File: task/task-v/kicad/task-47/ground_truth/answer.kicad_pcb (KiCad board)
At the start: 2 copper layers, 65 x 56.5 mm, 5 parts

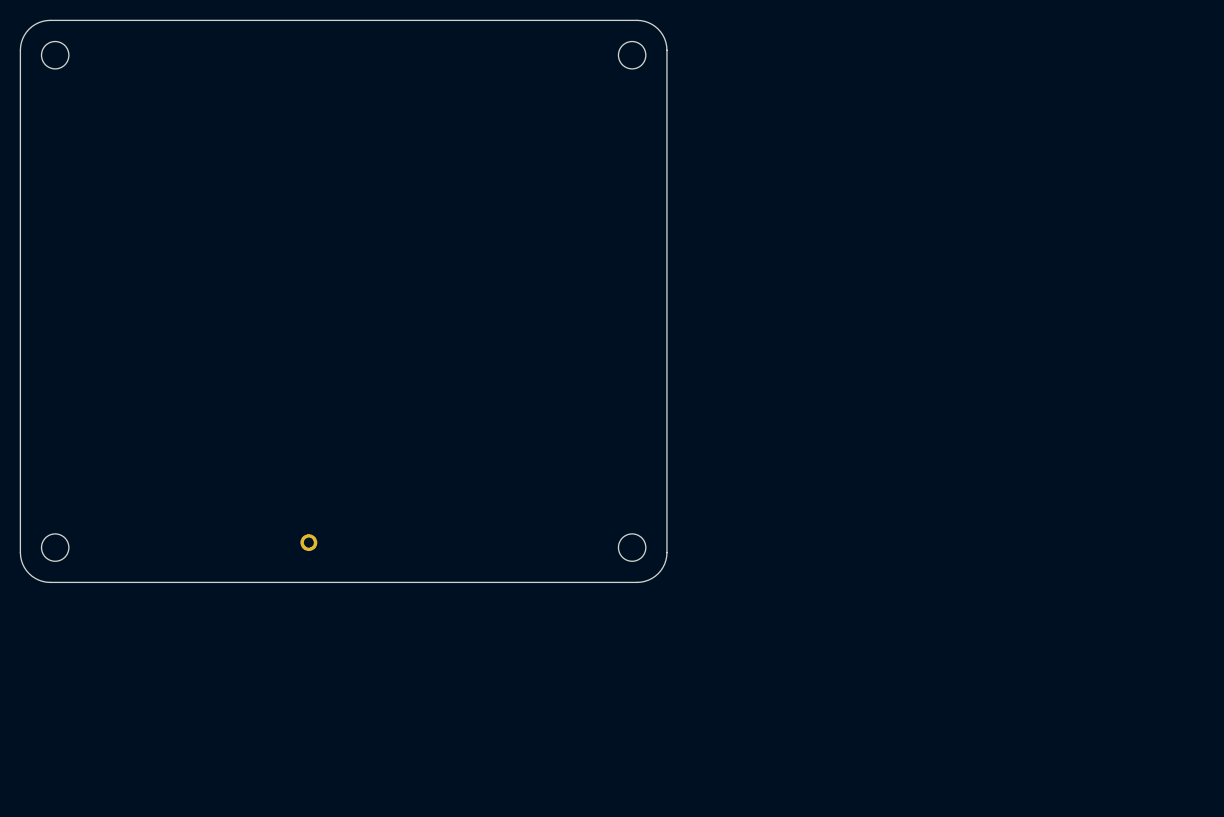
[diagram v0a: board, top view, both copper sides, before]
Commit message: Refine engineering task metadata and instructions
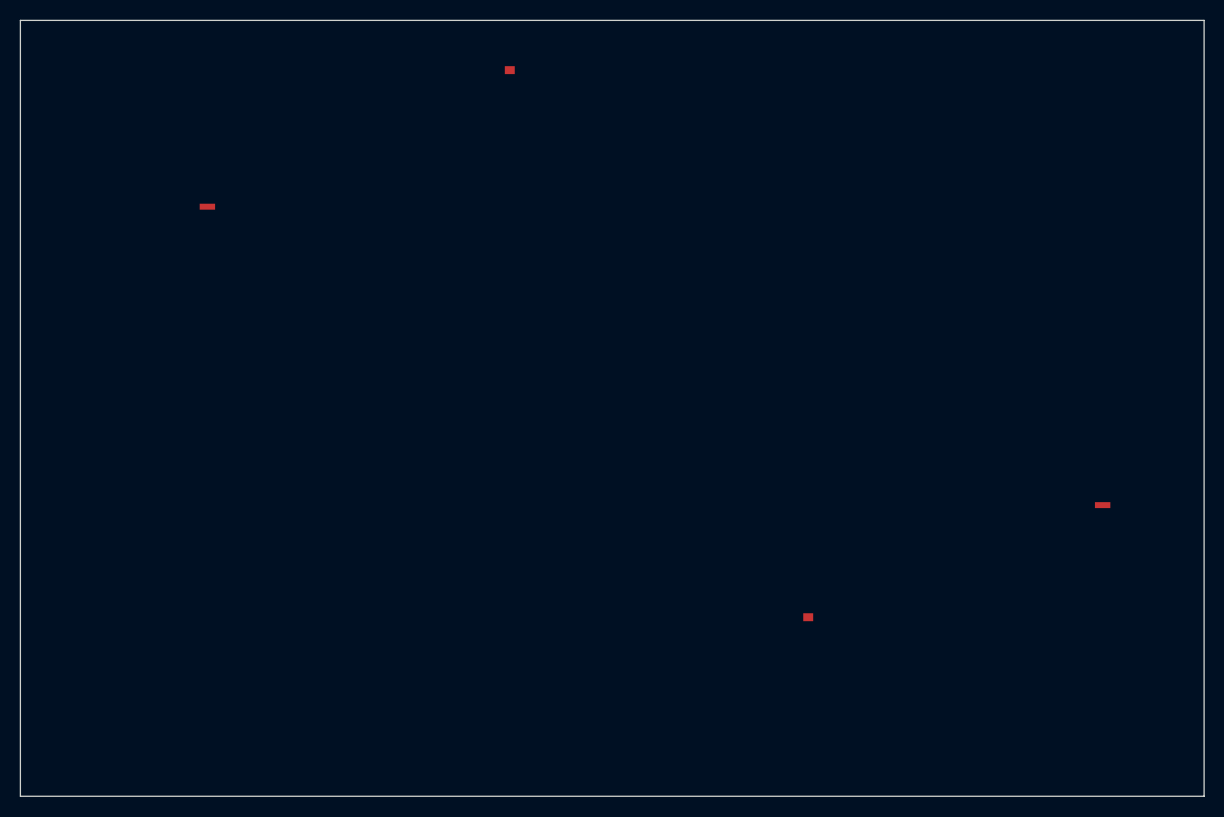
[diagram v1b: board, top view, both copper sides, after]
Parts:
- removed the ? at (3.50, 3.50)
- removed the ? at (61.5, 3.50)
- removed the ? at (3.50, 53.0)
- removed the ? at (61.5, 53.0)
- removed the ? at (29.0, 52.5)
- added ?: , Package_SO:SOIC-8_3.9x4.9mm_P1.27mm, F.Cu at (20.0, 20.0)
- added ?: , Resistor_SMD:R_0603_1608Metric, F.Cu at (50.0, 5.00)
- added ?: , Package_SO:SOIC-8_3.9x4.9mm_P1.27mm, F.Cu at (110.0, 50.0)
- added ?: , Resistor_SMD:R_0603_1608Metric, F.Cu at (80.0, 60.0)
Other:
- board size 65 x 56.5 mm -> 119 x 78 mm
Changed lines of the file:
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@@
   (net 1 "VCC")
   (net 2 "GND")
-  ; HAT+ board outline: 65x56.5mm with R=3mm rounded corners
-  ; Straight edges
-  (gr_line (start 3 0) (end 62 0) (layer "Edge.Cuts") (width 0.1))
-  (gr_line (start 65 3) (end 65 53.5) (layer "Edge.Cuts") (width 0.1))
-  (gr_line (start 62 56.5) (end 3 56.5) (layer "Edge.Cuts") (width 0.1))
-  (gr_line (start 0 53.5) (end 0 3) (layer "Edge.Cuts") (width 0.1))
-  ; Rounded corners (gr_arc: start, mid, end)
-  ; Bottom-left corner: center(3,3), R=3, arc from (0,3) through (0.879,0.879) to (3,0)
-  (gr_arc (start 0 3) (mid 0.879 0.879) (end 3 0) (layer "Edge.Cuts") (width 0.1))
-  ; Bottom-right corner: center(62,3), R=3, arc from (62,0) through (64.121,0.879) to (65,3)
-  (gr_arc (start 62 0) (mid 64.121 0.879) (end 65 3) (layer "Edge.Cuts") (width 0.1))
-  ; Top-right corner: center(62,53.5), R=3, arc from (65,53.5) through (64.121,55.621) to (62,56.5)
-  (gr_arc (start 65 53.5) (mid 64.121 55.621) (end 62 56.5) (layer "Edge.Cuts") (width 0.1))
-  ; Top-left corner: center(3,53.5), R=3, arc from (3,56.5) through (0.879,55.621) to (0,53.5)
-  (gr_arc (start 3 56.5) (mid 0.879 55.621) (end 0 53.5) (layer "Edge.Cuts") (width 0.1))
-  ; 4 M2.5 mounting holes at HAT+ spec positions
-  (footprint "MountingHole:MountingHole_2.75mm_M2.5" (layer "F.Cu") (at 3.5 3.5)
-    (reference "H1") (value "MountingHole")
-    (pad "" np_thru_hole circle (at 0 0) (size 2.75 2.75) (drill 2.75)
-      (layers "F.Cu" "B.Cu" "F.Mask" "B.Mask"))
+  ; Shrunk board: 119x78mm to fit Hammond 1455C1201 slot
+  (gr_rect (start 0 0) (end 119 78) (layer "Edge.Cuts") (width 0.1))
+  ; U1 at (20,20): dist to edges = min(20,99,20,58) = 20mm >= 3mm ✓
+  (footprint "Package_SO:SOIC-8_3.9x4.9mm_P1.27mm" (layer "F.Cu") (at 20 20)
+    (reference "U1") (value "OPAMP")
+    (pad "1" smd rect (at -1.2 -1.27) (size 1.55 0.6)
+      (layers "F.Cu" "F.Paste" "F.Mask") (net 1 "VCC"))
   )
-  (footprint "MountingHole:MountingHole_2.75mm_M2.5" (layer "F.Cu") (at 61.5 3.5)
-    (reference "H2") (value "MountingHole")
-    (pad "" np_thru_hole circle (at 0 0) (size 2.75 2.75) (drill 2.75)
-      (layers "F.Cu" "B.Cu" "F.Mask" "B.Mask"))
+  ; R1 moved from (50,1.5) to (50,5): dist to bottom edge = 5mm >= 3mm ✓
+  (footprint "Resistor_SMD:R_0603_1608Metric" (layer "F.Cu") (at 50 5)
+    (reference "R1") (value "4.7k")
+    (pad "1" smd rect (at -0.8 0) (size 1.0 0.8)
+      (layers "F.Cu" "F.Paste" "F.Mask") (net 1 "VCC"))
   )
-  (footprint "MountingHole:MountingHole_2.75mm_M2.5" (layer "F.Cu") (at 3.5 53)
-    (reference "H3") (value "MountingHole")
-    (pad "" np_thru_hole circle (at 0 0) (size 2.75 2.75) (drill 2.75)
-      (layers "F.Cu" "B.Cu" "F.Mask" "B.Mask"))
+  ; U2 moved from (148,50) to (110,50): dist to right edge (x=119) = 9mm >= 3mm ✓
+  (footprint "Package_SO:SOIC-8_3.9x4.9mm_P1.27mm" (layer "F.Cu") (at 110 50)
+    (reference "U2") (value "ADC")
+    (pad "1" smd rect (at -1.2 -1.27) (size 1.55 0.6)
+      (layers "F.Cu" "F.Paste" "F.Mask") (net 2 "GND"))
   )
-  (footprint "MountingHole:MountingHole_2.75mm_M2.5" (layer "F.Cu") (at 61.5 53)
-    (reference "H4") (value "MountingHole")
-    (pad "" np_thru_hole circle (at 0 0) (size 2.75 2.75) (drill 2.75)
-      (layers "F.Cu" "B.Cu" "F.Mask" "B.Mask"))
-  )
-  ; 2x20 GPIO header repositioned to HAT+ spec position (29.0, 52.5)
-  (footprint "Connector_PinHeader_2.54mm:PinHeader_2x20_P2.54mm_Vertical" (layer "F.Cu") (at 29.0 52.5)
-    (reference "J1") (value "GPIO_HEADER")
-    (pad "1" thru_hole circle (at 0 0) (size 1.7 1.7) (drill 1.0)
-      (layers "F.Cu" "B.Cu" "F.Mask" "B.Mask") (net 1 "VCC"))
+  ; R2 at (80,60): dist to edges = min(80,39,60,18) = 18mm >= 3mm ✓
+  (footprint "Resistor_SMD:R_0603_1608Metric" (layer "F.Cu") (at 80 60)
+    (reference "R2") (value "10k")
+    (pad "1" smd rect (at -0.8 0) (size 1.0 0.8)
+      (layers "F.Cu" "F.Paste" "F.Mask") (net 2 "GND"))
   )
 )
